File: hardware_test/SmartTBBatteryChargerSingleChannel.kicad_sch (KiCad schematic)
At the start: 103 parts, among them J1 XT60_MALE, J7 Conn_SWD, J8 Conn_01x02, Q1 BSC070N10NS5, U1 RY8411, U2 RS3236, U3 RY8411, U4 STM32G474RBTx, U5 INA240A1PW, U6 UCC27517, Y1 Crystal_GND24

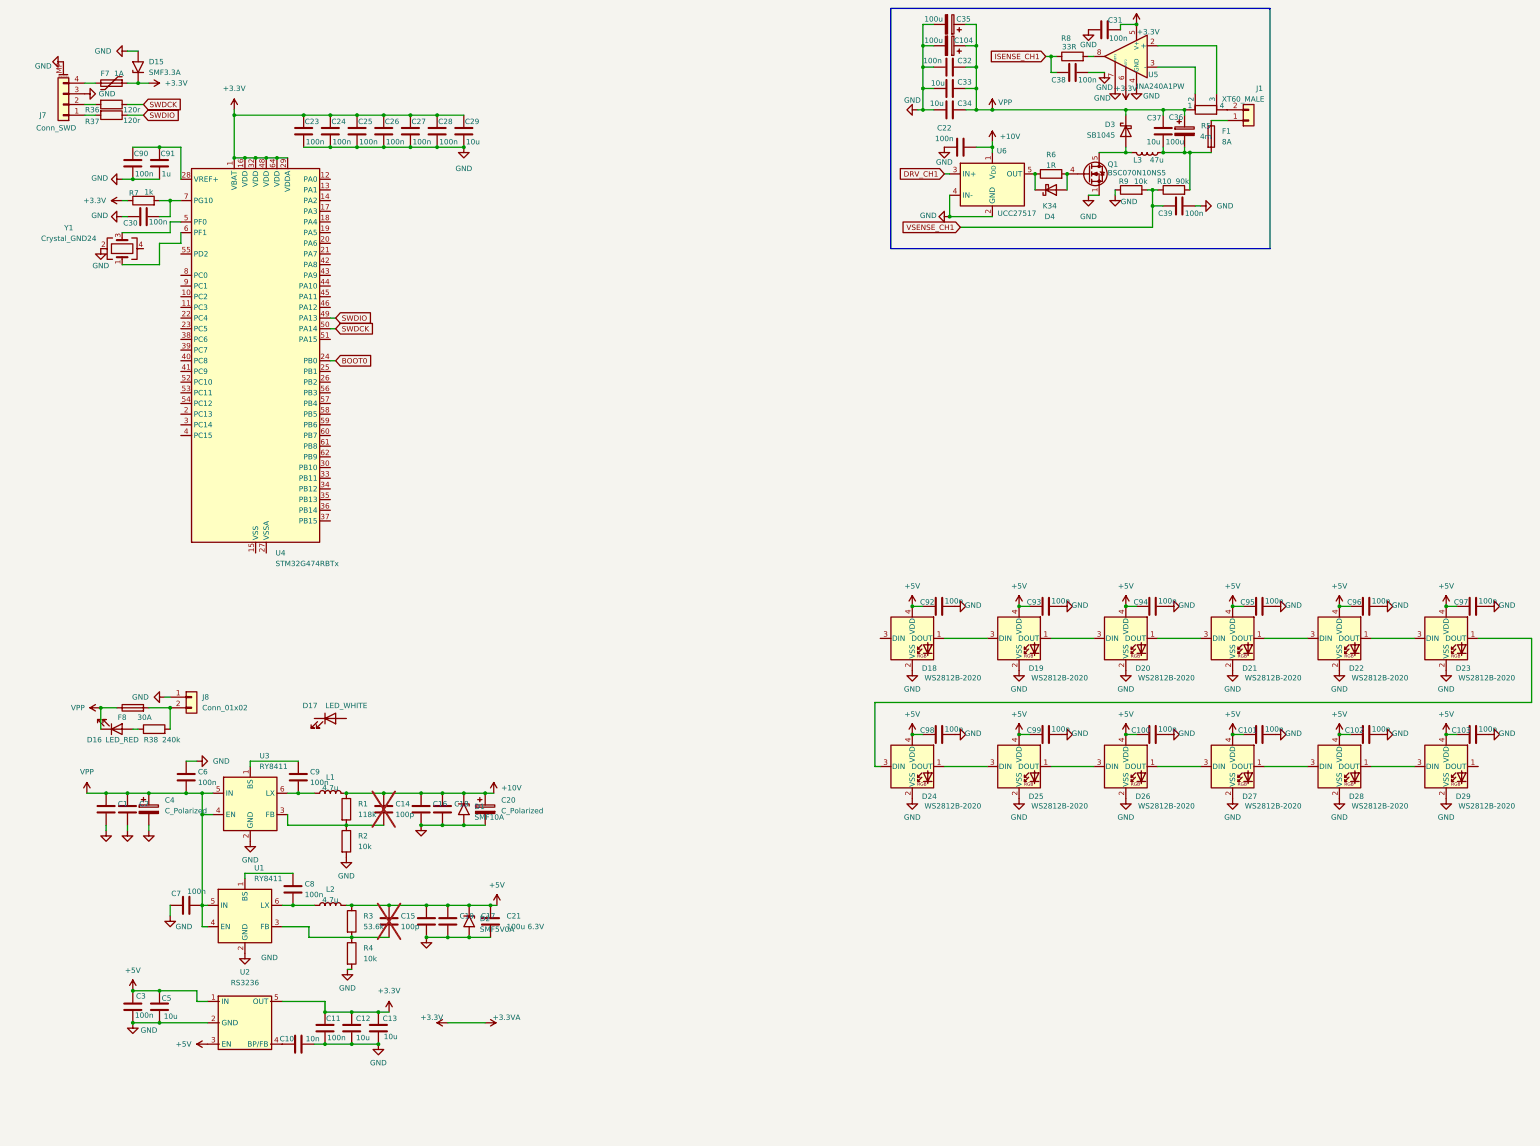
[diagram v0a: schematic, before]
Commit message: Test Hardware schematic done
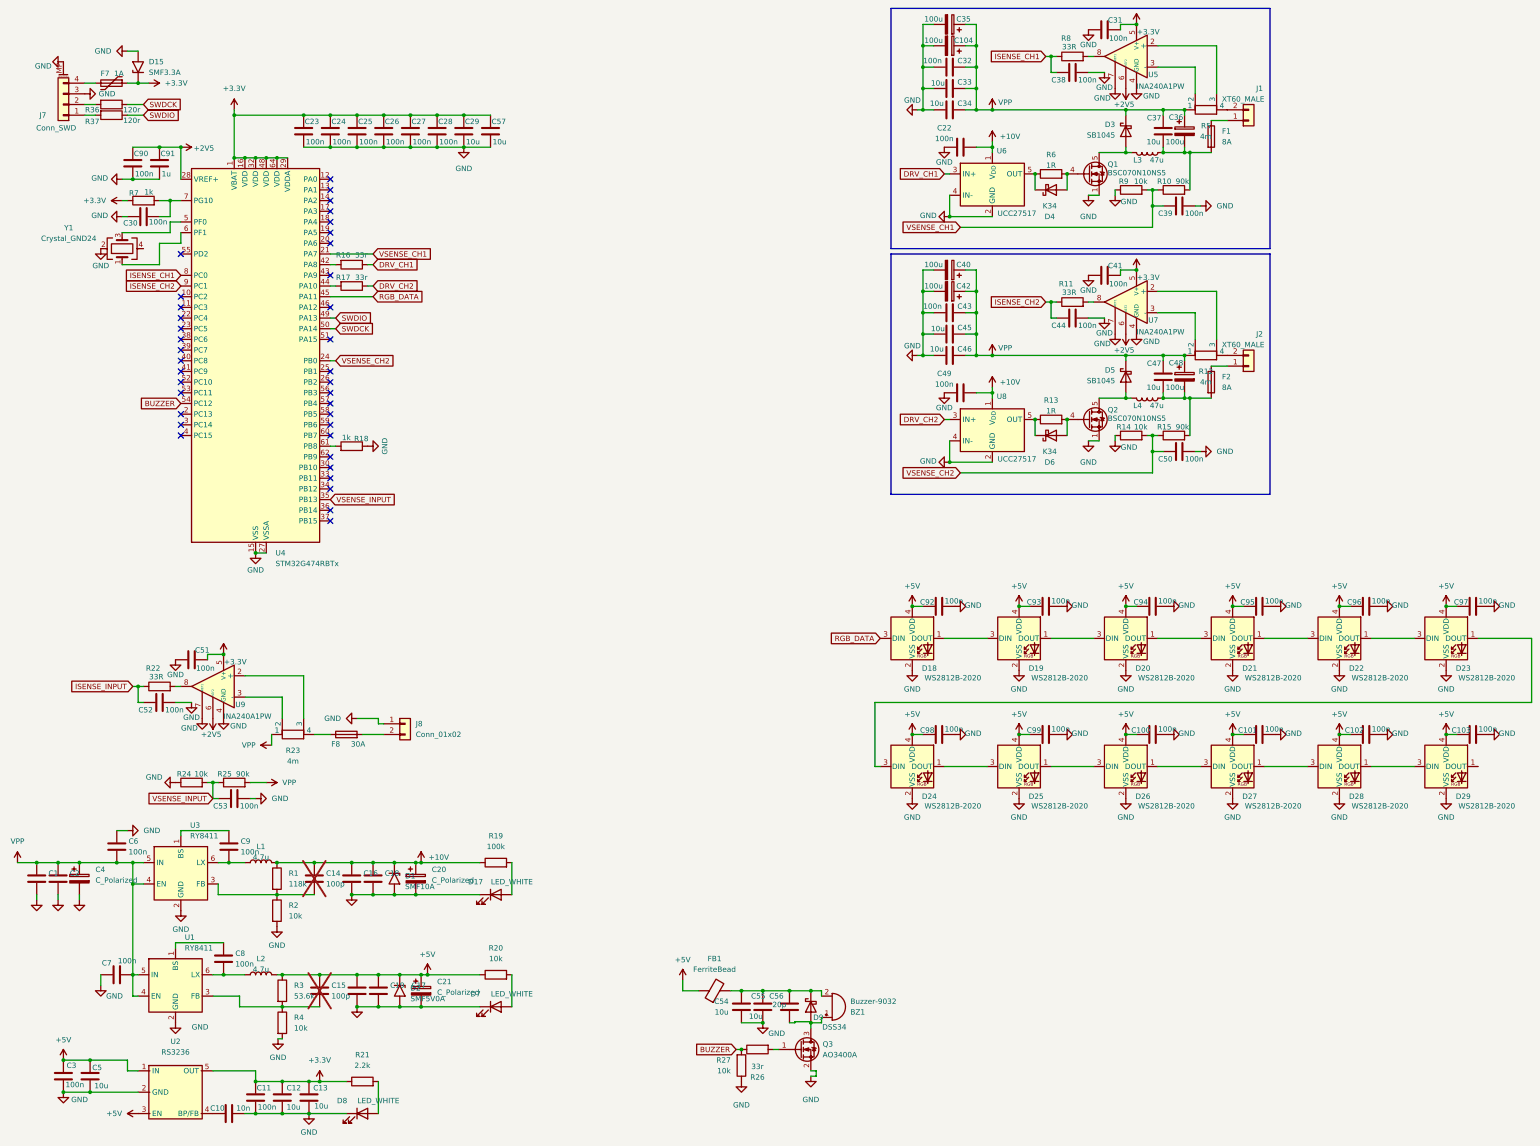
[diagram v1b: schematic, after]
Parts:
- removed C21: 100u 6.3V, Capacitor_SMD:C_1206_3216Metric, symbol Device:C
- removed D16: LED_RED, LED_SMD:LED_0603_1608Metric, symbol Device:LED
- removed R38: 240k, Resistor_SMD:R_0603_1608Metric, symbol Device:R
- added BZ1: Buzzer-9032, 0_RM2024:MLT-9032, symbol Device:Buzzer
- added C21: C_Polarized, Capacitor_THT:CP_Radial_D6.3mm_P2.50mm, symbol Device:C_Polarized
- added C40, C42, C48: 100u, Capacitor_THT:CP_Radial_D6.3mm_P2.50mm, symbol Device:C_Polarized
- added C41, C43, C44, C49, C50, C51, C52, C53: 100n, Capacitor_SMD:C_0603_1608Metric, symbol Device:C
- added C45, C46, C47: 10u, Capacitor_SMD:C_1206_3216Metric, symbol Device:C
- added C54, C55, C57: 10u, Capacitor_SMD:C_0603_1608Metric, symbol Device:C
- added C56: 20p, Capacitor_SMD:C_0603_1608Metric, symbol Device:C
- added D5: SB1045, Diode_SMD:D_PowerDI-5, symbol Device:D_Schottky
- added D6: K34, Diode_SMD:D_SOD-123F, symbol Device:D_Schottky
- added D7, D8: LED_WHITE, LED_SMD:LED_0603_1608Metric, symbol Device:LED
- added D9: DSS34, Diode_SMD:D_SMF, symbol Device:D_Schottky
- added F2: 8A, Fuse:Fuse_1206_3216Metric, symbol Device:Fuse
- added FB1: FerriteBead, Inductor_SMD:L_0603_1608Metric, symbol Device:FerriteBead
- added J2: XT60_MALE, Connector_AMASS:AMASS_XT60-M_1x02_P7.20mm_Vertical, symbol Connector_Generic:Conn_01x02
- added L4: 47u, Inductor_SMD:L_Coilcraft_MSS1260-XXX, symbol Device:L
- added Q2: BSC070N10NS5, Package_TO_SOT_SMD:TDSON-8-1, symbol Transistor_FET:BSC070N10NS5
- added Q3: AO3400A, Package_TO_SOT_SMD:SOT-23, symbol Transistor_FET:AO3400A
- added R11, R22: 33R, Resistor_SMD:R_0603_1608Metric, symbol Device:R
- added R12, R23: 4m, Resistor_SMD:R_Shunt_Vishay_WSK2512_6332Metric_T1.19mm, symbol Device:R_Shunt
- added R13: 1R, Resistor_SMD:R_0603_1608Metric, symbol Device:R
- added R14, R20, R24, R27: 10k, Resistor_SMD:R_0603_1608Metric, symbol Device:R
- added R15, R25: 90k, Resistor_SMD:R_0603_1608Metric, symbol Device:R
- added R16, R17, R26: 33r, Resistor_SMD:R_0603_1608Metric, symbol Device:R
- added R18: 1k, Resistor_SMD:R_0603_1608Metric, symbol Device:R
- added R19: 100k, Resistor_SMD:R_0603_1608Metric, symbol Device:R
- added R21: 2.2k, Resistor_SMD:R_0603_1608Metric, symbol Device:R
- added U7, U9: INA240A1PW, Package_SO:TSSOP-8_4.4x3mm_P0.65mm, symbol Amplifier_Current:INA240A1PW
- added U8: UCC27517, Package_TO_SOT_SMD:SOT-23-5, symbol 0_RM2024:UCC27517
- J8: footprint Connector_AMASS:AMASS_XT60PW-M_1x02_P7.20mm_Horizontal -> Connector_AMASS:AMASS_XT30U-M_1x02_P5.0mm_Vertical
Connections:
- net +10V: now also C49.1, R19.1, U8.1 (V_{DD})
- net +3.3V: now also C41.1, C51.1, C57.2, R21.1, U7.5 (V+), U9.5 (V+); no longer U5.6 (REF2)
- net +5V: now also C21.1, FB1.1, R20.1
- net DRV_CH1: now also R16.1
- net GND: now also D17.1 (K), U4.15 (VSS), U4.27 (VSSA), U4.31 (VSS), U4.47 (VSS), U4.63 (VSS), C21.2, C40.2, C41.2, C42.2, C43.2, C44.1, C45.2, C46.2, C49.2, C50.1, C51.2, C52.1, C53.1, C54.1, C55.1, C57.1, D7.1 (K), D8.1 (K), Q2.1 (S), Q2.2 (S), Q2.3 (S), Q3.2 (S), R14.1, R18.1, R24.1, R27.1, U7.1 (GND), U7.4 (GND), U7.7 (REF1), U8.2 (GND), U8.4 (IN-), U9.1 (GND), U9.4 (GND), U9.7 (REF1)
- net ISENSE_CH1: now also U4.8 (PC0)
- net VPP: now also C40.1, C42.1, C43.1, C45.1, C46.1, C47.1, C48.1, D5.1 (K), R12.1, R23.1, R25.2; no longer F8.1
- net VSENSE_CH1: now also U4.21 (PA7)
- net +2V5: now reaches C90.2, C91.2, U4.28 (VREF+)
- net +2V5: now also U5.6 (REF2), U7.6 (REF2), U9.6 (REF2)
- net VSENSE_INPUT: now reaches U4.35 (PB13)
- net VSENSE_INPUT: now also C53.2, R24.2, R25.1
- net at U4.42 (PA8): now also R16.2
- net at U4.44 (PA10): now also R17.2
- net RGB_DATA: now reaches U4.45 (PA11)
- net RGB_DATA: now also D18.3 (DIN)
- net BUZZER: now reaches U4.54 (PC12)
- net BUZZER: now also R26.1, R27.2
- net at U4.61 (PB8): now also R18.2
- net ISENSE_CH2: now reaches U4.9 (PC1)
- net ISENSE_CH2: now also C44.2, R11.1
- net at D17.2 (A): now also R19.2
- net BOOT0 renamed VSENSE_CH2
- net VSENSE_CH2: now also C50.2, R14.2, R15.1
- new net: F2.1, J2.1 (Pin_1)
- new net: J2.2 (Pin_2), R12.4
- new net: R11.2, U7.8
- new net: BZ1.2 (+), C54.2, C55.2, C56.2, D9.1 (K), FB1.2
- new net: BZ1.1 (-), C56.1, D9.2 (A), Q3.3 (D)
- new net: D6.1 (K), R13.1, U8.5 (OUT)
- new net: D7.2 (A), R20.2
- new net: D6.2 (A), Q2.4 (G), R13.2
- new net: C47.2, C48.2, F2.2, L4.2, R15.2
- new net: D5.2 (A), L4.1, Q2.5 (D)
- new net: R23.2, U9.3 (-)
- new net: R23.3, U9.2 (+)
- new net: F8.1, R23.4
- new net: Q3.1 (G), R26.2
- new net: R12.3, U7.2 (+)
- new net: R12.2, U7.3 (-)
- new net: D8.2 (A), R21.2
- new net: R22.2, U9.8
- new net DRV_CH2: R17.1, U8.3 (IN+)
- new net ISENSE_INPUT: C52.2, R22.1
- no-connect marks 0 -> 37
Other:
- moved on the sheet: C1, C10, C11, C12, C13, C14, C15, C16, C17, C18, C19, C2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

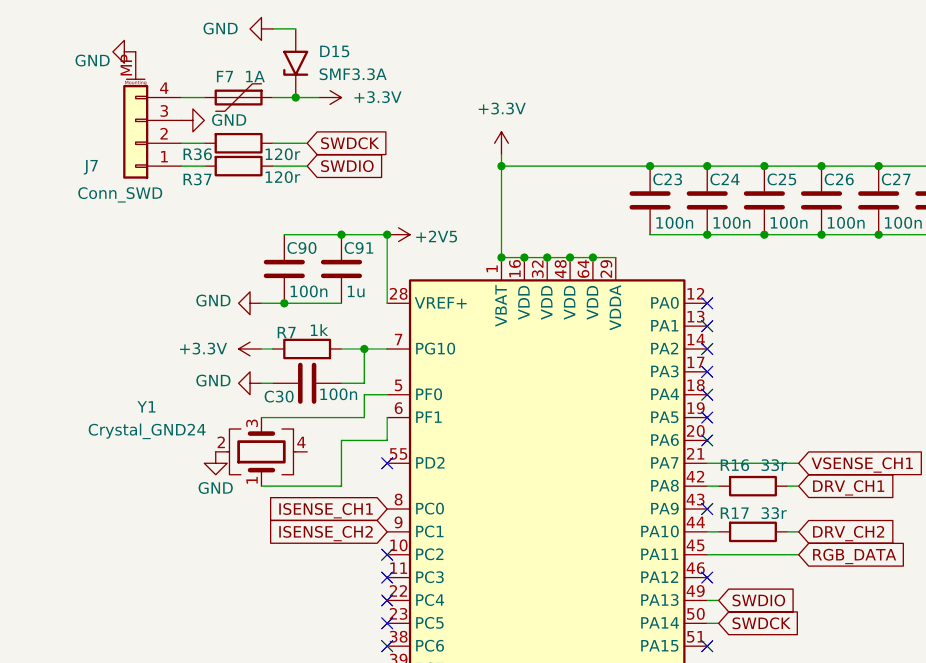
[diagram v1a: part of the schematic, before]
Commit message: Progress on hardware_test PCB
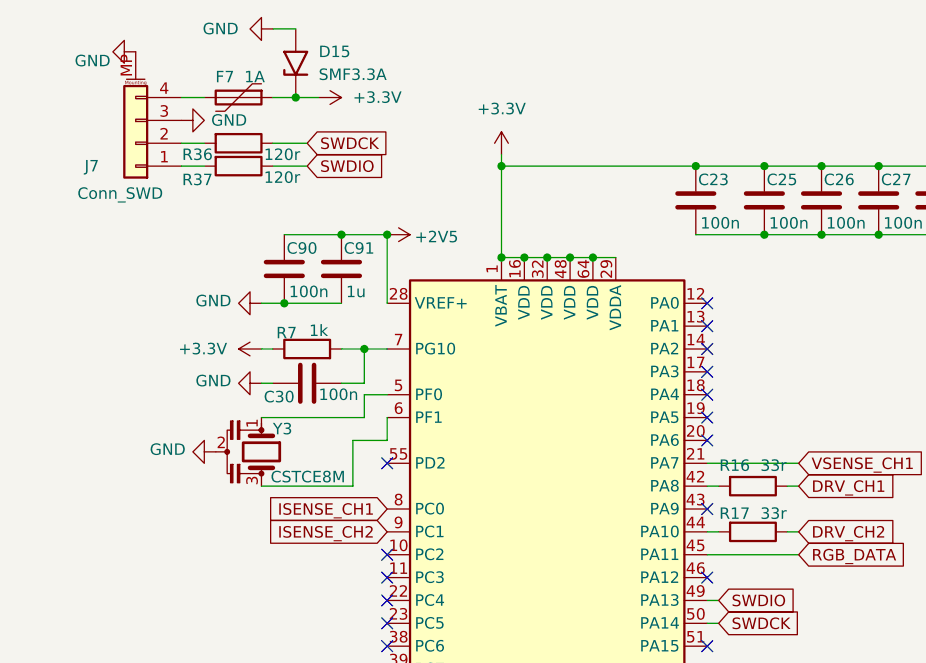
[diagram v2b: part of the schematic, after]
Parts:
- removed C24: 100n, Capacitor_SMD:C_0603_1608Metric, symbol Device:C
- removed Y1: Crystal_GND24, Crystal:Crystal_SMD_3225-4Pin_3.2x2.5mm, symbol Device:Crystal_GND24
- added Y3: CSTCE8M, Crystal:Resonator_SMD_Murata_CSTxExxV-3Pin_3.0x1.1mm_HandSoldering, symbol Device:Resonator
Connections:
- net GND: now also Y3.2
- net at U4.5 (PF0): now also Y3.1
- net at U4.6 (PF1): now also Y3.3
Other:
- moved on the sheet: C23

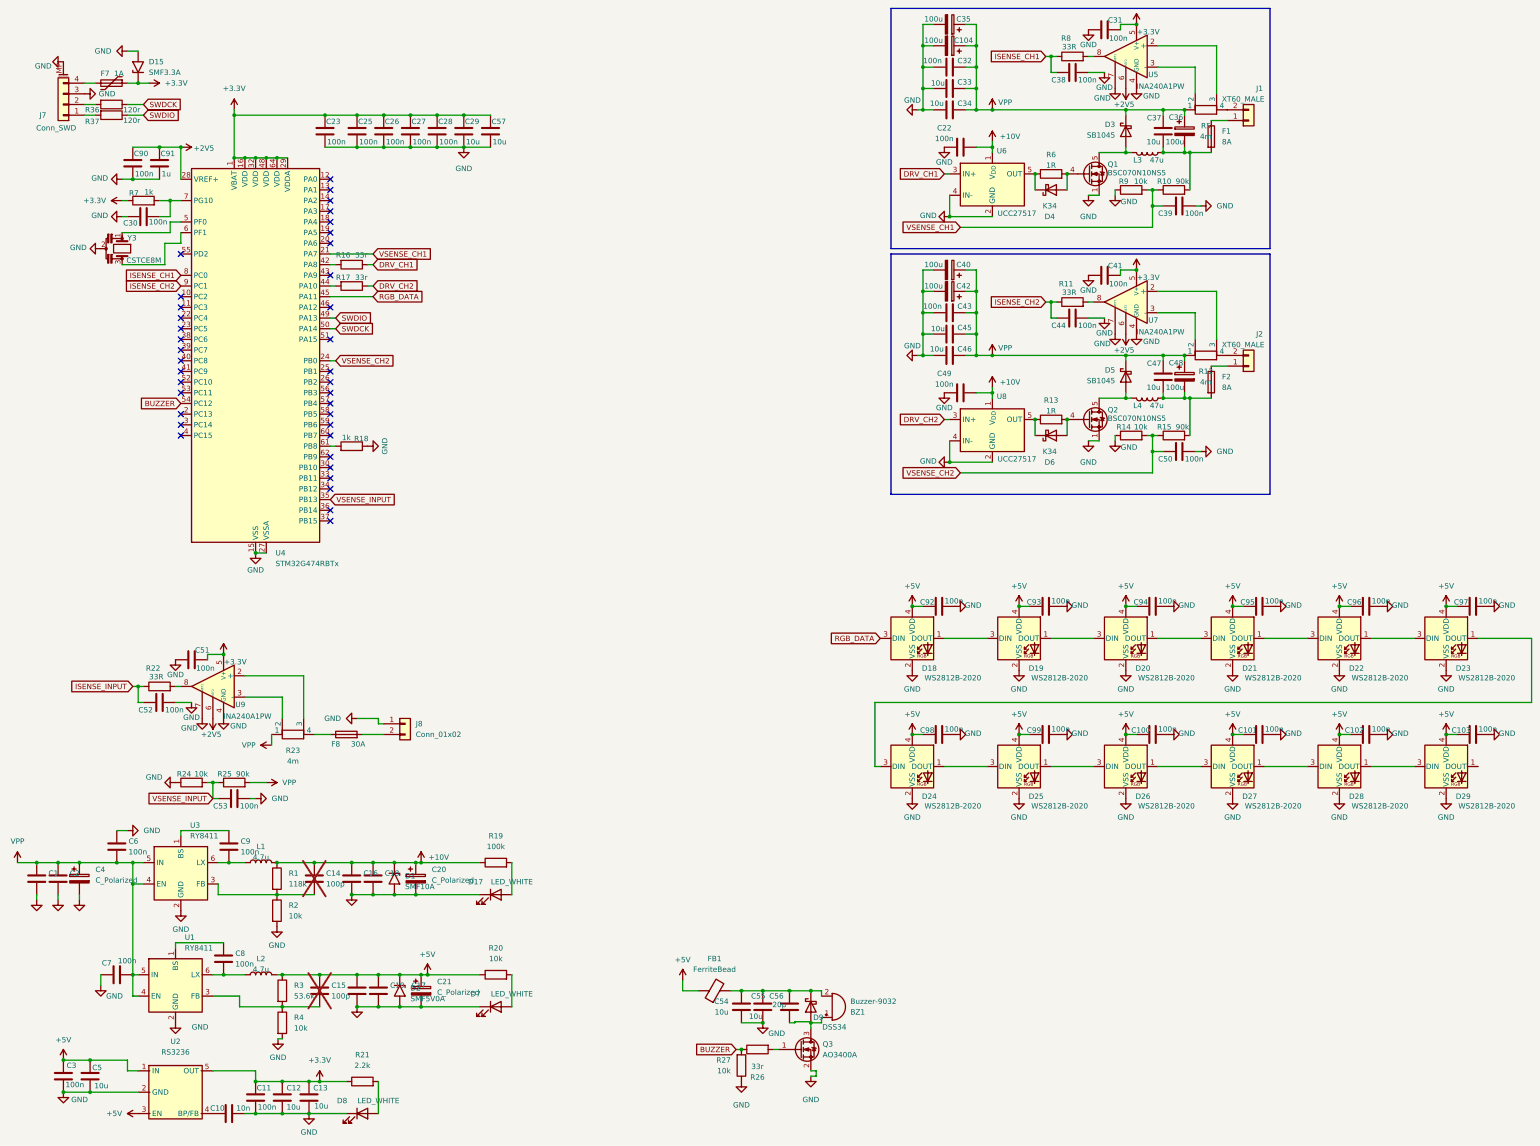
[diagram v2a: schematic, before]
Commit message: just more wiring...
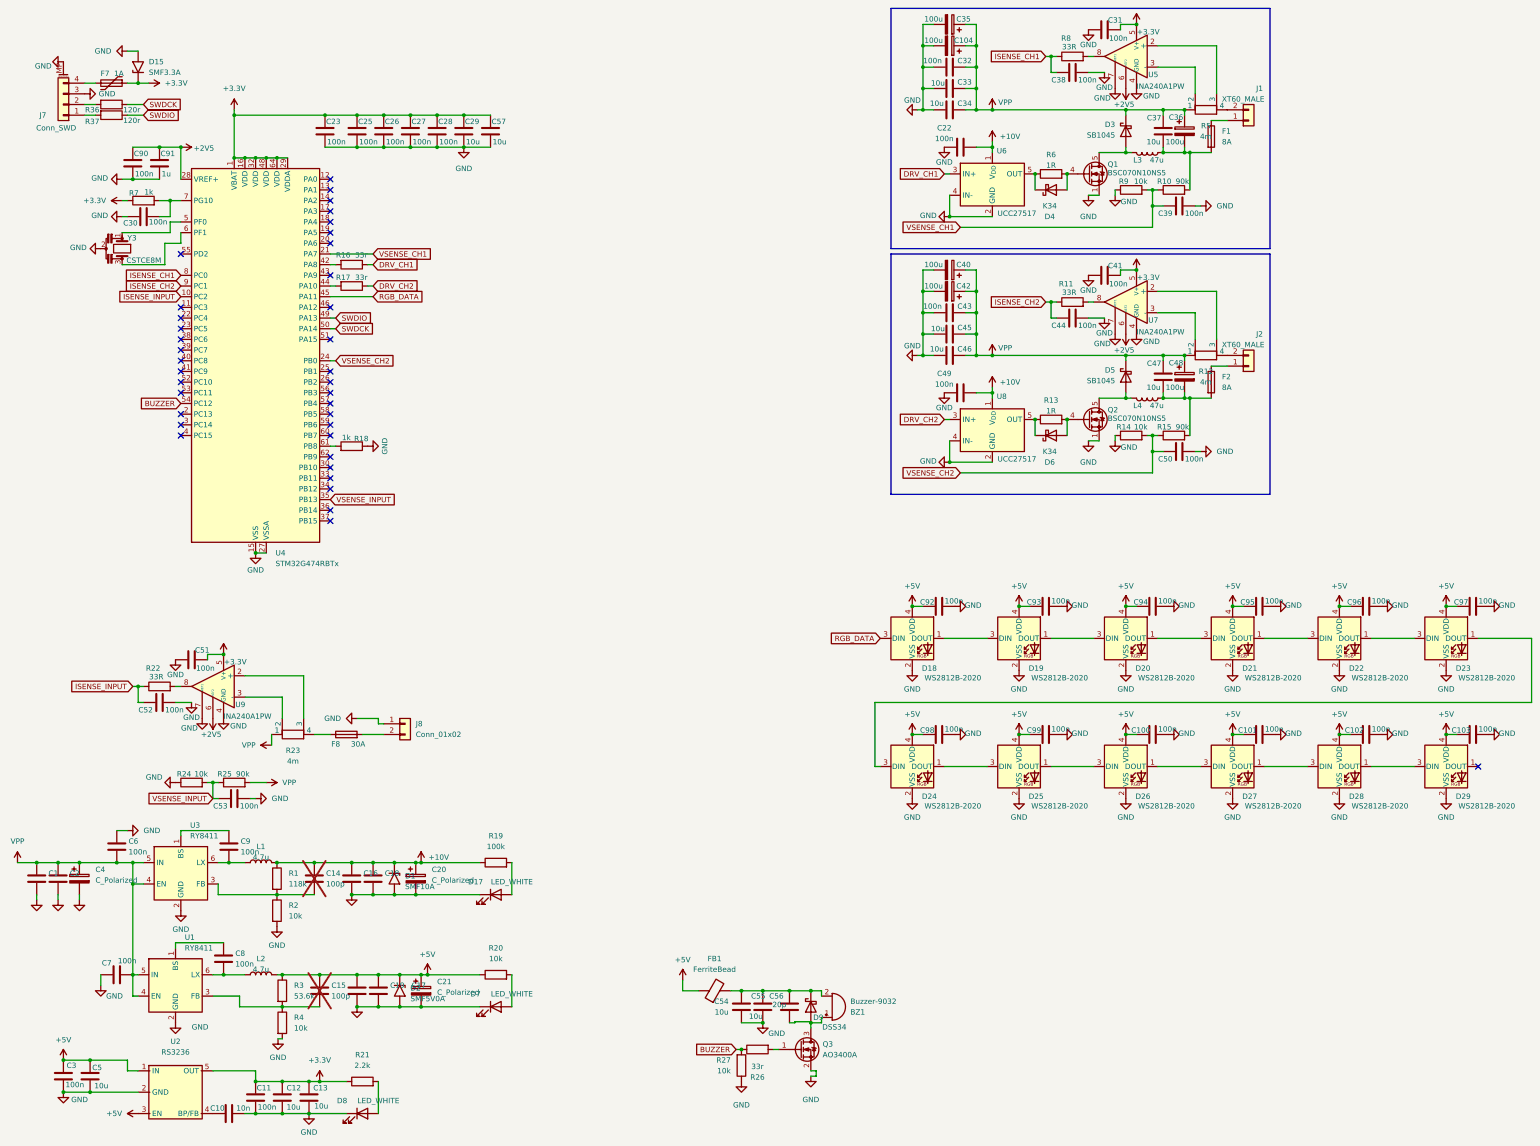
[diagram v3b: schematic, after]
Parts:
- BZ1: footprint 0_RM2024:MLT-9032 -> LinkedLibrary:MLT-9032
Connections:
- net ISENSE_INPUT: now also U4.10 (PC2)
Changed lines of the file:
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@@
 	)
 	(no_connect
-		(at 57.15 81.28)
-	)
-	(no_connect
 		(at 92.71 91.44)
 	)
@@
 	)
 	(no_connect
+		(at 365.76 193.04)
+	)
+	(no_connect
 		(at 92.71 101.6)
 	)
@@
 		)
 	)
+	(global_label "ISENSE_INPUT"
+		(shape input)
+		(at 57.15 81.28 180)
+		(fields_autoplaced yes)
+		(effects
+			(font
+				(size 1.27 1.27)
+			)
+			(justify right)
+		)
+		(property "Intersheetrefs" "${INTERSHEET_REFS}"
+			(at 41.0415 81.28 0)
+			(effects
+				(font
+					(size 1.27 1.27)
+				)
+				(justify right)
+				(hide yes)
+			)
+		)
+	)
 	(symbol
 		(lib_id "Device:C")
@@
 			)
 		)
-		(property "Footprint" "0_RM2024:MLT-9032"
+		(property "Footprint" "LinkedLibrary:MLT-9032"
 			(at 211.455 252.73 90)
 			(effects
